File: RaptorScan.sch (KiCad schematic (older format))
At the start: 1 part

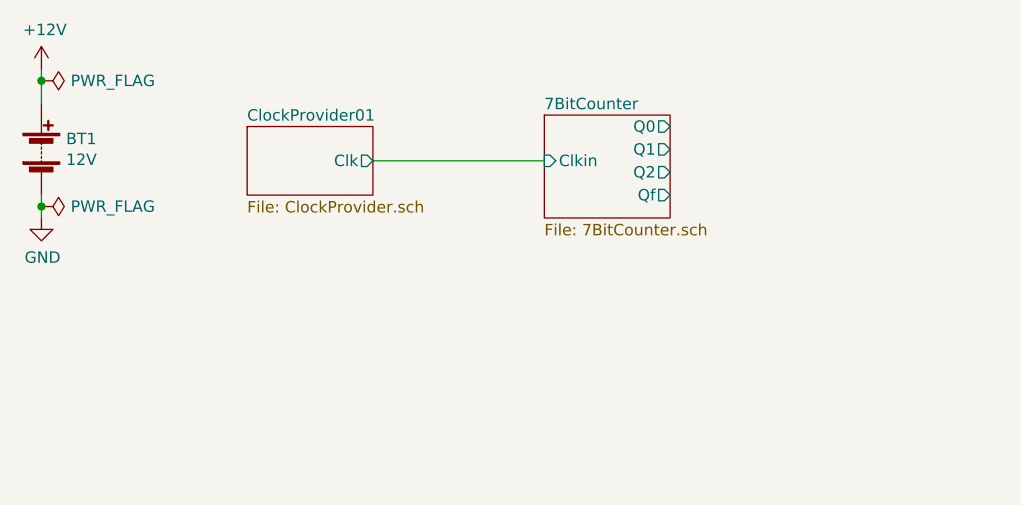
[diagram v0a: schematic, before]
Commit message: Update
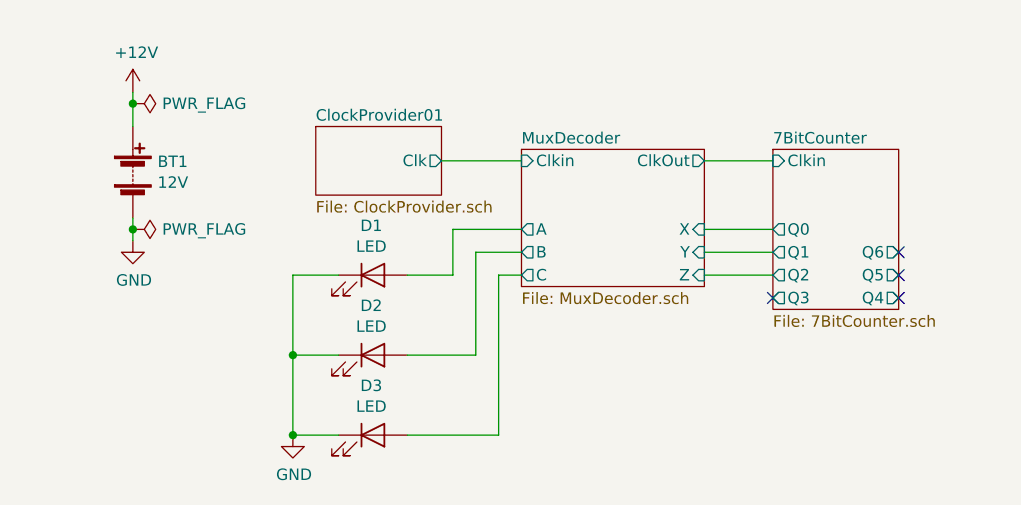
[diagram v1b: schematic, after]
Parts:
- added D1, D2, D3: LED, symbol Device:LED
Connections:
- net GND: now also D1.1 (K), D2.1 (K), D3.1 (K)
- new net MuxDecoder/A: D1.2 (A)
- new net MuxDecoder/B: D2.2 (A)
- new net MuxDecoder/C: D3.2 (A)
- no-connect marks 0 -> 4
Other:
- moved on the sheet: BT1
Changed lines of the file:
@@
 $Descr A4 11693 8268
 encoding utf-8
-Sheet 1 3
+Sheet 1 4
 Title ""
 Date ""
@@
 $EndDescr
 $Sheet
-S 2000 950  550  300
+S 2300 950  550  300
 U 5D1172DE
 F0 "ClockProvider01" 50
 F1 "ClockProvider.sch" 50
-F2 "Clk" O R 2550 1100 50
+F2 "Clk" O R 2850 1100 50
 $EndSheet
 Wire Wire Line
-	1100 700  1100 750
+	1500 800  1500 850
 $Comp
 L power:+12V #PWR0102
 U 1 1 5D1362F3
-P 1100 700
-F 0 "#PWR0102" H 1100 550 50  0001 C CNN
-F 1 "+12V" H 1115 873 50  0000 C CNN
-F 2 "" H 1100 700 50  0001 C CNN
-F 3 "" H 1100 700 50  0001 C CNN
-	1    1100 700
+P 1500 800
+F 0 "#PWR0102" H 1500 650 50  0001 C CNN
+F 1 "+12V" H 1515 973 50  0000 C CNN
+F 2 "" H 1500 800 50  0001 C CNN
+F 3 "" H 1500 800 50  0001 C CNN
+	1    1500 800
 	1    0    0    -1
 $EndComp
@@
 L power:GND #PWR0103
 U 1 1 5D137CC7
-P 1100 1350
-F 0 "#PWR0103" H 1100 1100 50  0001 C CNN
-F 1 "GND" H 1105 1177 50  0000 C CNN
-F 2 "" H 1100 1350 50  0001 C CNN
-F 3 "" H 1100 1350 50  0001 C CNN
-	1    1100 1350
-	1    0    0    -1
-$EndComp
-Wire Wire Line
-	1100 1250 1100 1300
+P 1500 1450
+F 0 "#PWR0103" H 1500 1200 50  0001 C CNN
+F 1 "GND" H 1505 1277 50  0000 C CNN
+F 2 "" H 1500 1450 50  0001 C CNN
+F 3 "" H 1500 1450 50  0001 C CNN
+	1    1500 1450
+	1    0    0    -1
+$EndComp
+Wire Wire Line
+	1500 1350 1500 1400
 $Comp
 L power:PWR_FLAG #FLG0101
 U 1 1 5D13C6DB
-P 1100 750
-F 0 "#FLG0101" H 1100 825 50  0001 C CNN
-F 1 "PWR_FLAG" V 1100 878 50  0000 L CNN
-F 2 "" H 1100 750 50  0001 C CNN
-F 3 "~" H 1100 750 50  0001 C CNN
-	1    1100 750
+P 1500 850
+F 0 "#FLG0101" H 1500 925 50  0001 C CNN
+F 1 "PWR_FLAG" V 1500 978 50  0000 L CNN
+F 2 "" H 1500 850 50  0001 C CNN
+F 3 "~" H 1500 850 50  0001 C CNN
+	1    1500 850
 	0    1    1    0
 $EndComp
-Connection ~ 1100 750
-Wire Wire Line
-	1100 750  1100 850
+Connection ~ 1500 850
+Wire Wire Line
+	1500 850  1500 950
 $Comp
 L power:PWR_FLAG #FLG0102
 U 1 1 5D13CBD4
-P 1100 1300
-F 0 "#FLG0102" H 1100 1375 50  0001 C CNN
-F 1 "PWR_FLAG" V 1100 1428 50  0000 L CNN
-F 2 "" H 1100 1300 50  0001 C CNN
-F 3 "~" H 1100 1300 50  0001 C CNN
-	1    1100 1300
+P 1500 1400
+F 0 "#FLG0102" H 1500 1475 50  0001 C CNN
+F 1 "PWR_FLAG" V 1500 1528 50  0000 L CNN
+F 2 "" H 1500 1400 50  0001 C CNN
+F 3 "~" H 1500 1400 50  0001 C CNN
+	1    1500 1400
 	0    1    1    0
 $EndComp
-Connection ~ 1100 1300
-Wire Wire Line
-	1100 1300 1100 1350
+Connection ~ 1500 1400
+Wire Wire Line
+	1500 1400 1500 1450
 $Comp
 L Device:Battery BT1
 U 1 1 5D11AF0F
-P 1100 1050
-F 0 "BT1" H 1208 1096 50  0000 L CNN
-F 1 "12V" H 1208 1005 50  0000 L CNN
-F 2 "" V 1100 1110 50  0001 C CNN
-F 3 "~" V 1100 1110 50  0001 C CNN
-	1    1100 1050
+P 1500 1150
+F 0 "BT1" H 1608 1196 50  0000 L CNN
+F 1 "12V" H 1608 1105 50  0000 L CNN
+F 2 "" V 1500 1210 50  0001 C CNN
+F 3 "~" V 1500 1210 50  0001 C CNN
+	1    1500 1150
 	1    0    0    -1
 $EndComp
 $Sheet
-S 3300 900  550  450
+S 4300 1050 550  700
 U 5D12D5A5
 F0 "7BitCounter" 50
 F1 "7BitCounter.sch" 50
-F2 "Clkin" I L 3300 1100 50
-F3 "Q0" O R 3850 950 50
-F4 "Q1" O R 3850 1050 50
-F5 "Q2" O R 3850 1150 50
-F6 "Qf" O R 3850 1250 50
+F2 "Clkin" I L 4300 1100 50
+F3 "Q0" O L 4300 1400 50
+F4 "Q1" O L 4300 1500 50
+F5 "Q2" O L 4300 1600 50
+F6 "Q3" O L 4300 1700 50
+F7 "Q4" O R 4850 1700 50
+F8 "Q5" O R 4850 1600 50
+F9 "Q6" O R 4850 1500 50
 $EndSheet
-Wire Wire Line
-	2550 1100 3300 1100
+$Sheet
+S 3200 1050 800  600
+U 5D12D28E
+F0 "MuxDecoder" 50
+F1 "MuxDecoder.sch" 50
+F2 "A" O L 3200 1400 50
+F3 "B" O L 3200 1500 50
+F4 "C" O L 3200 1600 50
+F5 "X" I R 4000 1400 50
+F6 "Y" I R 4000 1500 50
+F7 "Z" I R 4000 1600 50
+F8 "Clkin" I L 3200 1100 50
+F9 "ClkOut" O R 4000 1100 50
+$EndSheet
+Wire Wire Line
+	4300 1400 4000 1400
+Wire Wire Line
+	4300 1500 4000 1500
+Wire Wire Line
+	4300 1600 4000 1600
+NoConn ~ 4300 1700
+Wire Wire Line
+	2850 1100 3200 1100
+Wire Wire Line
+	4000 1100 4300 1100
+NoConn ~ 4850 1500
+NoConn ~ 4850 1600
+NoConn ~ 4850 1700
+$Comp
+L Device:LED D1
+U 1 1 5D23D3BD
+P 2550 1600
+F 0 "D1" H 2543 1816 50  0000 C CNN
+F 1 "LED" H 2543 1725 50  0000 C CNN
+F 2 "" H 2550 1600 50  0001 C CNN
+F 3 "~" H 2550 1600 50  0001 C CNN
+	1    2550 1600
+	1    0    0    -1
+$EndComp
+$Comp
+L Device:LED D2
+U 1 1 5D23E2F8
+P 2550 1950
+F 0 "D2" H 2543 2166 50  0000 C CNN
+F 1 "LED" H 2543 2075 50  0000 C CNN
+F 2 "" H 2550 1950 50  0001 C CNN
+F 3 "~" H 2550 1950 50  0001 C CNN
+	1    2550 1950
+	1    0    0    -1
+$EndComp
+$Comp
+L Device:LED D3
+U 1 1 5D23E6C2
+P 2550 2300
+F 0 "D3" H 2543 2516 50  0000 C CNN
+F 1 "LED" H 2543 2425 50  0000 C CNN
+F 2 "" H 2550 2300 50  0001 C CNN
+F 3 "~" H 2550 2300 50  0001 C CNN
+	1    2550 2300
+	1    0    0    -1
+$EndComp
+Wire Wire Line
+	2700 1600 2900 1600
+Wire Wire Line
+	2900 1600 2900 1400
+Wire Wire Line
+	2900 1400 3200 1400
+Wire Wire Line
+	3200 1500 3000 1500
+Wire Wire Line
+	3000 1500 3000 1950
+Wire Wire Line
+	3000 1950 2700 1950
+Wire Wire Line
+	3200 1600 3100 1600
+Wire Wire Line
+	3100 1600 3100 2300
+Wire Wire Line
+	3100 2300 2700 2300
+Wire Wire Line
+	2400 2300 2200 2300
+Wire Wire Line
+	2200 2300 2200 1950
+Wire Wire Line
+	2200 1600 2400 1600
+Wire Wire Line
+	2400 1950 2200 1950
+Connection ~ 2200 1950
+Wire Wire Line
+	2200 1950 2200 1600
+$Comp
+L power:GND #PWR0104
+U 1 1 5D23FAED
+P 2200 2300
+F 0 "#PWR0104" H 2200 2050 50  0001 C CNN
+F 1 "GND" H 2205 2127 50  0000 C CNN
+F 2 "" H 2200 2300 50  0001 C CNN
+F 3 "" H 2200 2300 50  0001 C CNN
+	1    2200 2300
+	1    0    0    -1
+$EndComp
+Connection ~ 2200 2300
 $EndSCHEMATC
